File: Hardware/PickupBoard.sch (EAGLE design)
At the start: 29 parts, among them U1 TL074_

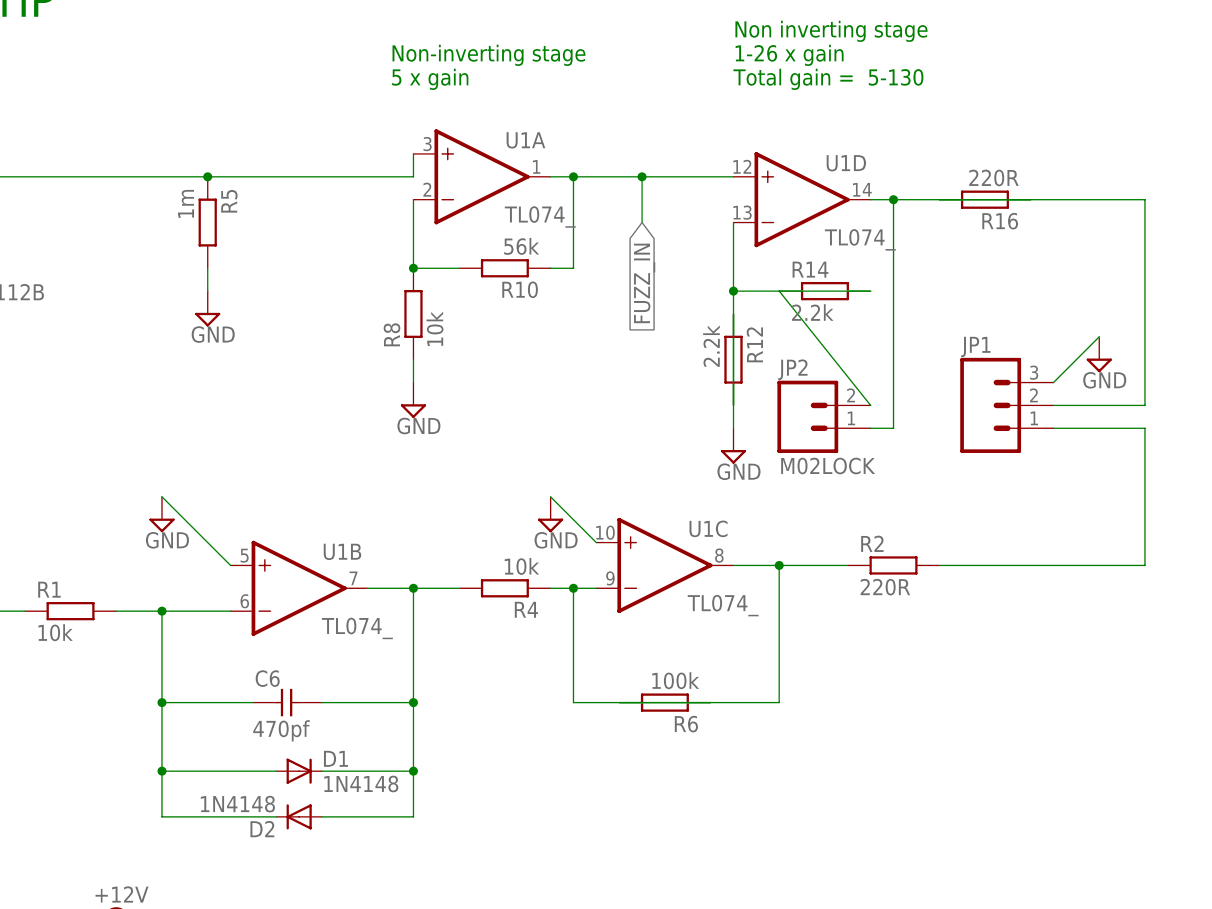
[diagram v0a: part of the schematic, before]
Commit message: Rev 4 pcb
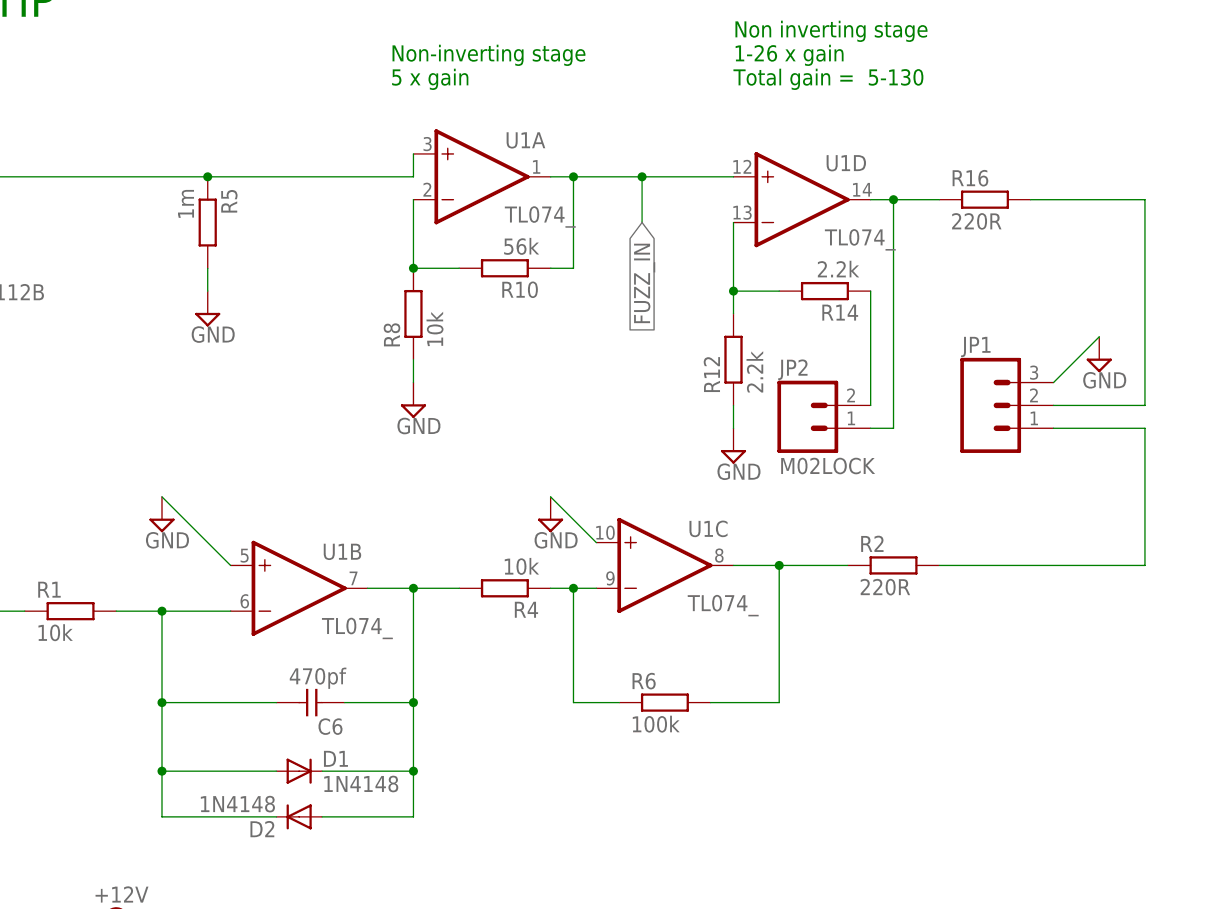
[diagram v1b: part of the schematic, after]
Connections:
- net N$2: now also C6.2; no longer C6.1
- net N$4: now also C6.1; no longer C6.2
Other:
- moved on the sheet: C6, R12, R14, R16, R6
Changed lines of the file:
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@@
 <?xml version="1.0" encoding="utf-8"?>
 <!DOCTYPE eagle SYSTEM "eagle.dtd">
-<eagle version="7.4.0">
+<eagle version="7.2.0">
 <drawing>
 <settings>
@@
 <instance part="R5" gate="G$1" x="99.06" y="121.92" rot="R270"/>
 <instance part="SUPPLY4" gate="GND" x="99.06" y="111.76"/>
-<instance part="R14" gate="G$1" x="167.64" y="114.3"/>
-<instance part="R16" gate="G$1" x="185.42" y="124.46" rot="R180"/>
+<instance part="R14" gate="G$1" x="167.64" y="114.3" rot="R180"/>
+<instance part="R16" gate="G$1" x="185.42" y="124.46"/>
 <instance part="R8" gate="G$1" x="121.92" y="111.76" rot="R90"/>
 <instance part="R10" gate="G$1" x="132.08" y="116.84" rot="R180"/>
 <instance part="SUPPLY9" gate="GND" x="121.92" y="101.6"/>
-<instance part="R12" gate="G$1" x="157.48" y="106.68" rot="R270"/>
+<instance part="R12" gate="G$1" x="157.48" y="106.68" rot="R90"/>
 <instance part="SUPPLY5" gate="GND" x="157.48" y="96.52"/>
 <instance part="GND21" gate="1" x="76.2" y="27.94"/>
@@
 <instance part="D1" gate="G$1" x="109.22" y="60.96"/>
 <instance part="D2" gate="G$1" x="109.22" y="55.88" rot="R180"/>
-<instance part="C6" gate="G$1" x="109.22" y="68.58" rot="R270"/>
+<instance part="C6" gate="G$1" x="109.22" y="68.58" rot="R90"/>
 <instance part="R4" gate="G$1" x="132.08" y="81.28" rot="R180"/>
 <instance part="SUPPLY2" gate="GND" x="137.16" y="88.9"/>
-<instance part="R6" gate="G$1" x="149.86" y="68.58" rot="R180"/>
+<instance part="R6" gate="G$1" x="149.86" y="68.58"/>
 </instances>
 <busses>
@@
 <pinref part="R12" gate="G$1" pin="1"/>
 <pinref part="SUPPLY5" gate="GND" pin="GND"/>
-<wire x1="157.48" y1="111.76" x2="157.48" y2="99.06" width="0.1524" layer="91"/>
+<wire x1="157.48" y1="101.6" x2="157.48" y2="99.06" width="0.1524" layer="91"/>
 </segment>
 <segment>
@@
 <segment>
 <pinref part="U1" gate="D" pin="OUT"/>
-<wire x1="190.5" y1="124.46" x2="175.26" y2="124.46" width="0.1524" layer="91"/>
+<wire x1="180.34" y1="124.46" x2="175.26" y2="124.46" width="0.1524" layer="91"/>
 <wire x1="175.26" y1="124.46" x2="172.72" y2="124.46" width="0.1524" layer="91"/>
 <pinref part="R16" gate="G$1" pin="1"/>
@@
 <segment>
 <pinref part="R16" gate="G$1" pin="2"/>
-<wire x1="203.2" y1="124.46" x2="180.34" y2="124.46" width="0.1524" layer="91"/>
+<wire x1="203.2" y1="124.46" x2="190.5" y2="124.46" width="0.1524" layer="91"/>
 <wire x1="203.2" y1="124.46" x2="203.2" y2="101.6" width="0.1524" layer="91"/>
 <pinref part="JP1" gate="G$1" pin="2"/>
@@
 <pinref part="R12" gate="G$1" pin="2"/>
 <pinref part="R14" gate="G$1" pin="2"/>
-<wire x1="157.48" y1="114.3" x2="157.48" y2="101.6" width="0.1524" layer="91"/>
-<wire x1="172.72" y1="114.3" x2="157.48" y2="114.3" width="0.1524" layer="91"/>
+<wire x1="157.48" y1="114.3" x2="157.48" y2="111.76" width="0.1524" layer="91"/>
+<wire x1="162.56" y1="114.3" x2="157.48" y2="114.3" width="0.1524" layer="91"/>
 <junction x="157.48" y="114.3"/>
 </segment>
@@
 <segment>
 <pinref part="R14" gate="G$1" pin="1"/>
-<wire x1="162.56" y1="114.3" x2="172.72" y2="101.6" width="0.1524" layer="91"/>
+<wire x1="172.72" y1="114.3" x2="172.72" y2="101.6" width="0.1524" layer="91"/>
 <pinref part="JP2" gate="G$1" pin="2"/>
 </segment>
@@
 <wire x1="93.98" y1="55.88" x2="93.98" y2="60.96" width="0.1524" layer="91"/>
 <junction x="93.98" y="60.96"/>
-<pinref part="C6" gate="G$1" pin="2"/>
-<wire x1="104.14" y1="68.58" x2="93.98" y2="68.58" width="0.1524" layer="91"/>
+<pinref part="C6" gate="G$1" pin="1"/>
+<wire x1="106.68" y1="68.58" x2="93.98" y2="68.58" width="0.1524" layer="91"/>
 <junction x="93.98" y="68.58"/>
 </segment>
@@
 <wire x1="121.92" y1="55.88" x2="121.92" y2="60.96" width="0.1524" layer="91"/>
 <junction x="121.92" y="60.96"/>
-<pinref part="C6" gate="G$1" pin="1"/>
-<wire x1="111.76" y1="68.58" x2="121.92" y2="68.58" width="0.1524" layer="91"/>
+<pinref part="C6" gate="G$1" pin="2"/>
+<wire x1="114.3" y1="68.58" x2="121.92" y2="68.58" width="0.1524" layer="91"/>
 <junction x="121.92" y="68.58"/>
 <pinref part="R4" gate="G$1" pin="2"/>
@@
 <pinref part="R6" gate="G$1" pin="1"/>
 <wire x1="139.7" y1="81.28" x2="137.16" y2="81.28" width="0.1524" layer="91"/>
-<wire x1="154.94" y1="68.58" x2="139.7" y2="68.58" width="0.1524" layer="91"/>
+<wire x1="144.78" y1="68.58" x2="139.7" y2="68.58" width="0.1524" layer="91"/>
 <wire x1="139.7" y1="68.58" x2="139.7" y2="81.28" width="0.1524" layer="91"/>
 <junction x="139.7" y="81.28"/>
@@
 <pinref part="R6" gate="G$1" pin="2"/>
 <wire x1="162.56" y1="83.82" x2="157.48" y2="83.82" width="0.1524" layer="91"/>
-<wire x1="144.78" y1="68.58" x2="162.56" y2="68.58" width="0.1524" layer="91"/>
+<wire x1="154.94" y1="68.58" x2="162.56" y2="68.58" width="0.1524" layer="91"/>
 <wire x1="162.56" y1="68.58" x2="162.56" y2="83.82" width="0.1524" layer="91"/>
 <junction x="162.56" y="83.82"/>

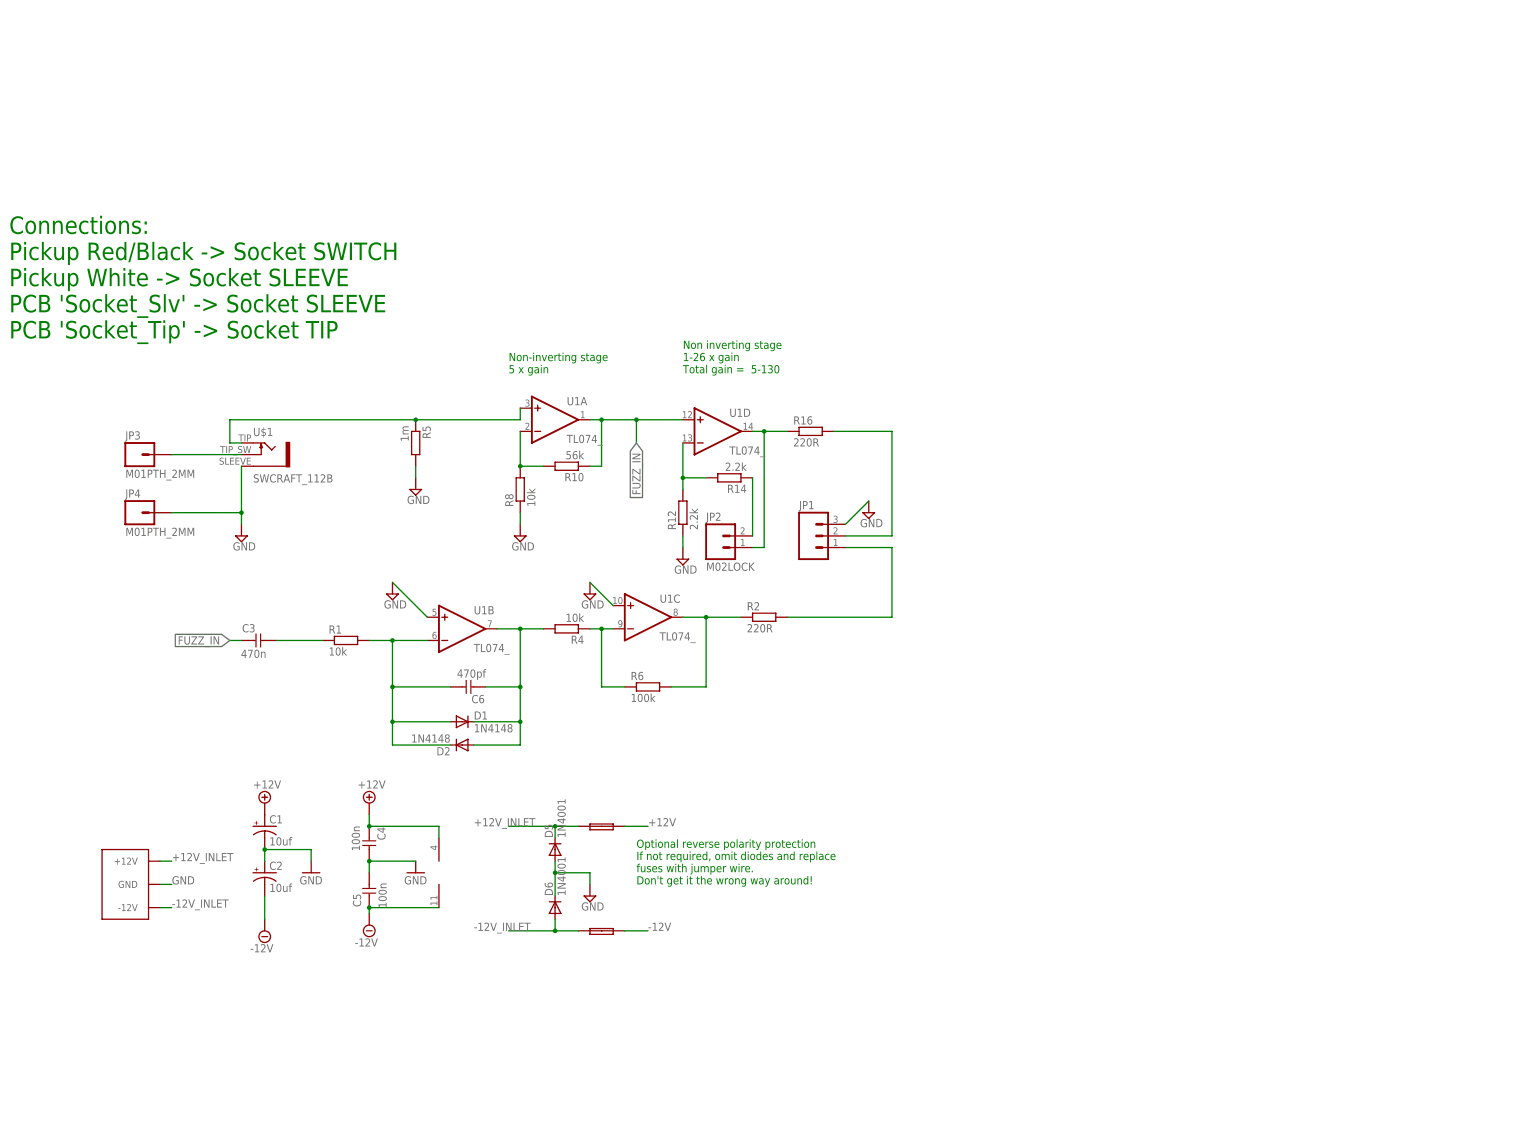
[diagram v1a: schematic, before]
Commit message: First rev5 upload
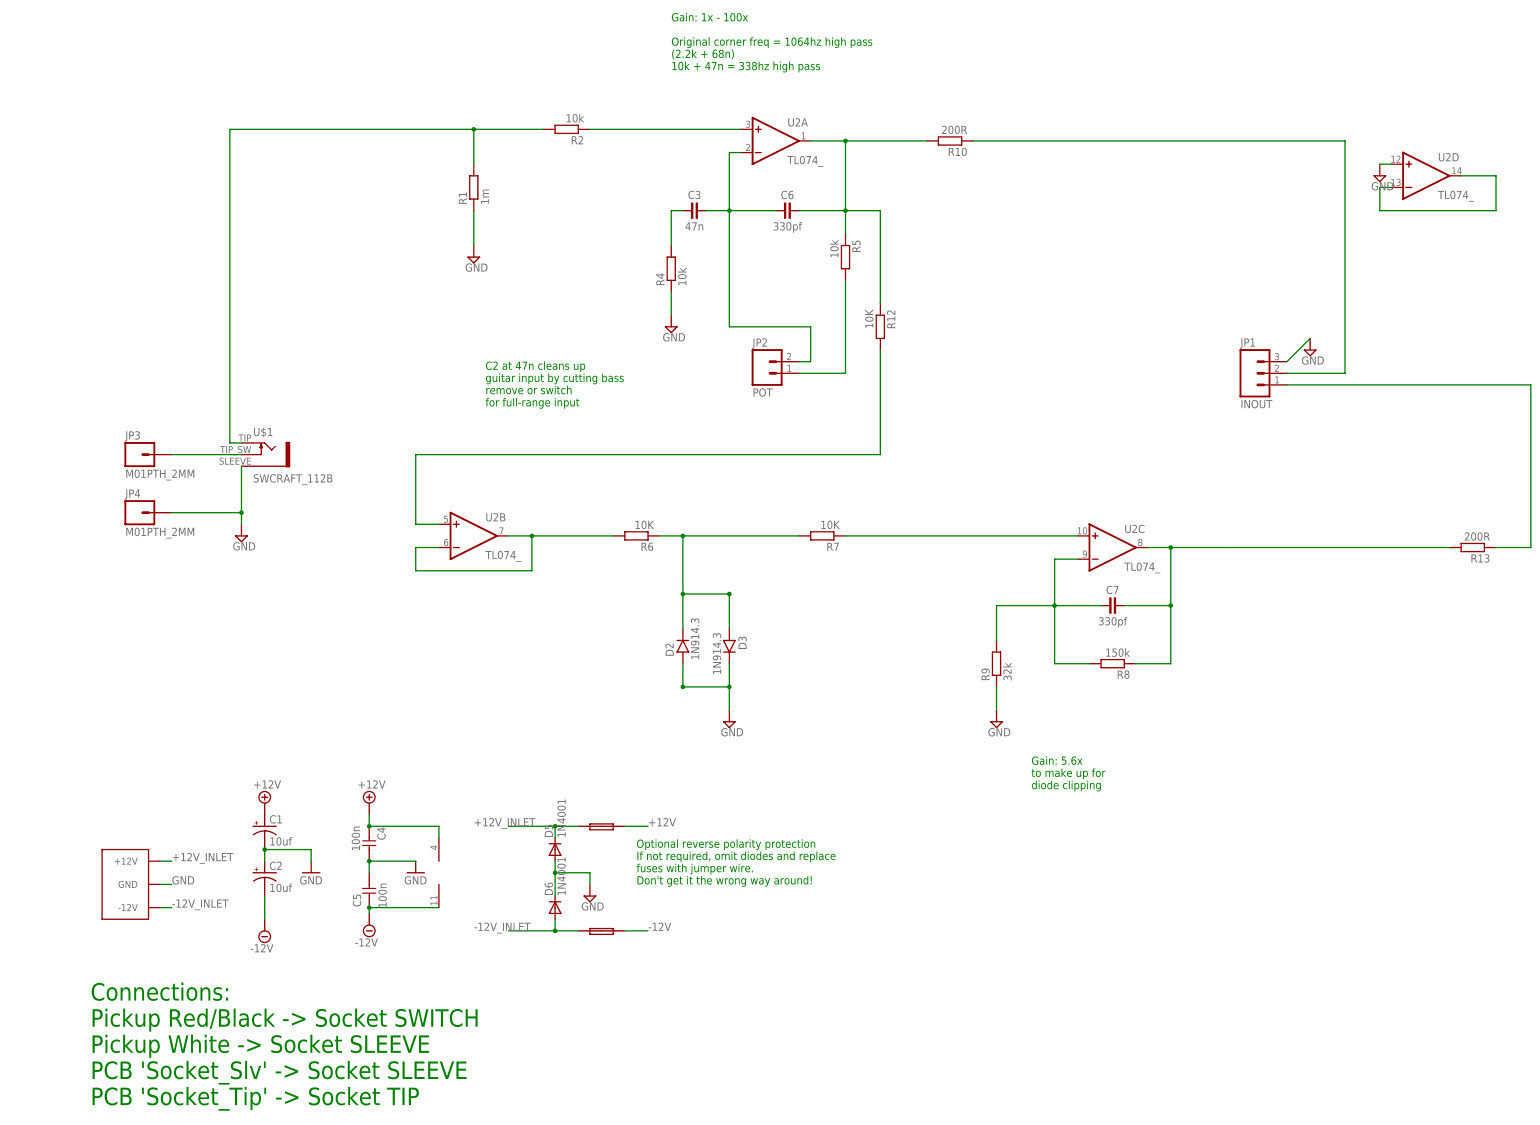
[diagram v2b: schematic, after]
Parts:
- removed D1: 1N4148, MusicThingModular:SMALL_DIODEDO35-7
- removed R14: 2.2k, MusicThingModular:RESISTOR7MM
- removed R16: 220R, MusicThingModular:RESISTOR7MM
- removed U1: TL074_, MusicThingModular:TL074_
- added C7: 330pf, we-rcl:CAPACITOR-0603
- added D3: 1N914.3, gm-diodes:1N914.3
- added R13: 200R, MusicThingModular:RESISTOR7MM
- added R7: 10K, MusicThingModular:RESISTOR7MM
- added R9: 32k, MusicThingModular:RESISTOR7MM
- added U2: TL074_, MusicThingModular:TL074_
- C3: value 470n -> 47n; device TomW:C-EU050-024X044 -> we-rcl:CAPACITOR-0603
- C6: value 470pf -> 330pf; device TomW:C-EU050-024X044 -> we-rcl:CAPACITOR-0603
- D2: value 1N4148 -> 1N914.3; device MusicThingModular:SMALL_DIODEDO35-7 -> gm-diodes:1N914.3
- JP1: value (none) -> INOUT
- JP2: value M02LOCK -> POT
- R1: value 10k -> 1m
- R10: value 56k -> 200R
- R12: value 2.2k -> 10K
- R2: value 220R -> 10k
- R5: value 1m -> 10k
- R6: value 100k -> 10K
- R8: value 10k -> 150k
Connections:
- removed net FUZZ_IN: C3.2, R10.1, U1A.OUT, U1D.+IN
- removed net N$1: R5.1, U$1.3, U1A.+IN
- removed net N$10: JP1.2, R16.2
- removed net N$5: JP2.2, R14.1
- new net GAIN_IN: R1.2, R2.2, U$1.3
- new net N$12: C7.2, R8.1, U2C.OUT
- new net N$15: C6.2, R10.2, R12.1, R5.1, U2A.OUT
- new net N$16: JP1.2, R10.1
- new net N$17: R12.2, U2B.+IN
- new net N$18: R6.2, U2B.-IN, U2B.OUT
- new net N$19: JP1.1, R13.1
- net +12V: now also U2P.V+; no longer U1P.V+
- net -12V: now also U2P.V-; no longer U1P.V-
- net GND: now also D2.A, D3.C, R1.1, R4.1, R9.1, U2D.+IN; no longer R12.1, R5.2, R8.1, U1B.+IN, U1C.+IN
- net N$11: now also C7.1, R8.2, R9.2, U2C.-IN; no longer R2.1, R6.2, U1C.OUT
- net N$13: now also R13.2; no longer JP1.1, R2.2
- net N$2: now also R2.1, U2A.+IN; no longer C6.2, D1.C, D2.A, R4.2, U1B.OUT
- net N$3: now also U2D.-IN, U2D.OUT; no longer R10.2, R8.2, U1A.-IN
- net N$4: now also C3.2, JP2.2, U2A.-IN; no longer D1.A, D2.C, R1.2, U1B.-IN
- net N$6: now also JP2.1, R5.2; no longer R12.2, R14.2, U1D.-IN
- net N$7: now also R4.2; no longer R1.1
- net N$8: now also R7.1, U2C.+IN; no longer JP2.1, R16.1, U1D.OUT
- net N$9: now also D2.C, D3.A, R7.2; no longer R4.1, U1C.-IN
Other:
- note added: "C2 at 47n cleans up guitar input by cutting bass remove or switch for full-range input"
- note added: "Gain: 1x - 100x Original corner freq = 1064hz high pass (2.2k + 68n) 10k + 47n = 338hz high pass"
- note added: "Gain: 5.6x to make up for diode clipping"
- note removed: "Non inverting stage 1-26 x gain Total gain = 5-130"
- note removed: "Non-inverting stage 5 x gain"
- moved on the sheet: D2, JP1, JP2, R1, R10, R12, R2, R4, R5, R6, R8
